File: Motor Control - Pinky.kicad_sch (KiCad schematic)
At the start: 9 parts, among them J4 BM09B-SRSS-TB, U12 TB9051FTG,EL

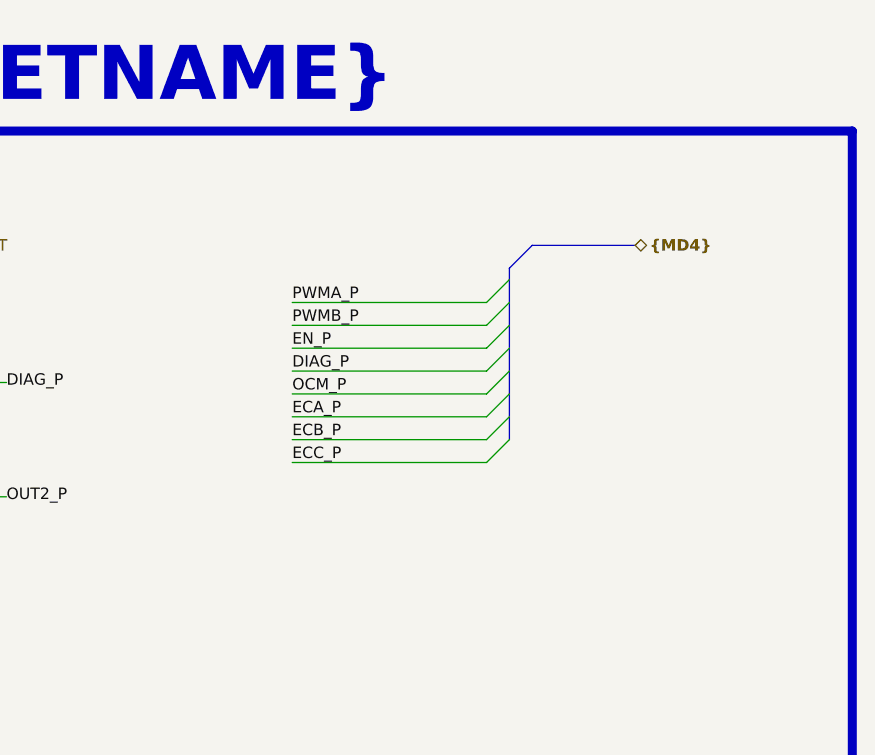
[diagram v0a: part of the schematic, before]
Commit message: Update Schematic
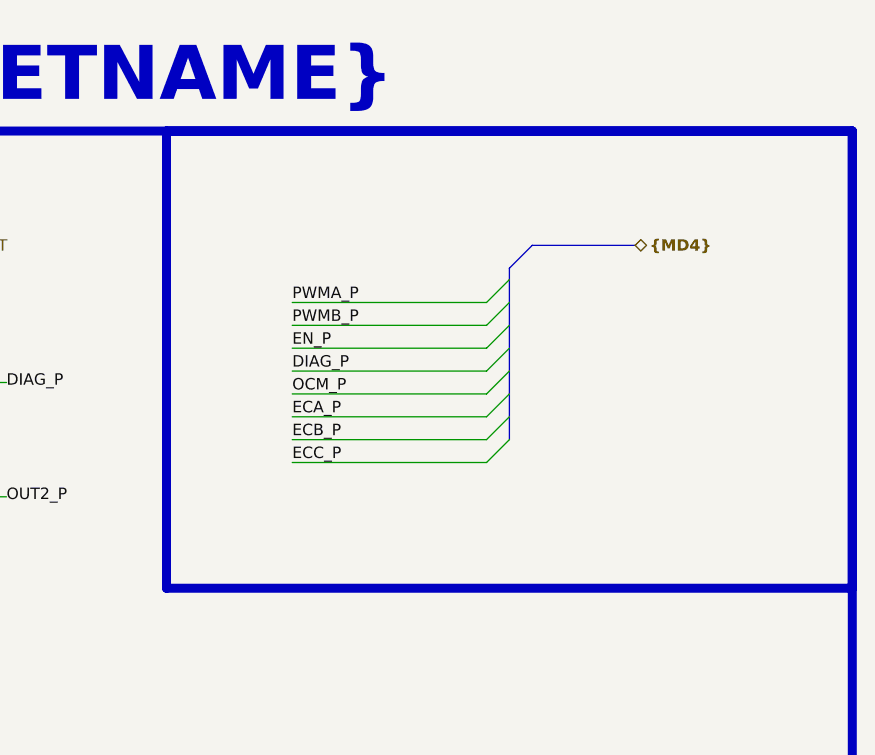
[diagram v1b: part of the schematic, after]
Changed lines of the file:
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@@
+		)
+	)
+	(rectangle
+		(start 177.8 25.4)
+		(end 254 76.2)
+		(stroke
+			(width 1)
+			(type default)
+			(color 200 0 0 1)
+		)
+		(fill
+			(type none)
 		)
 	)

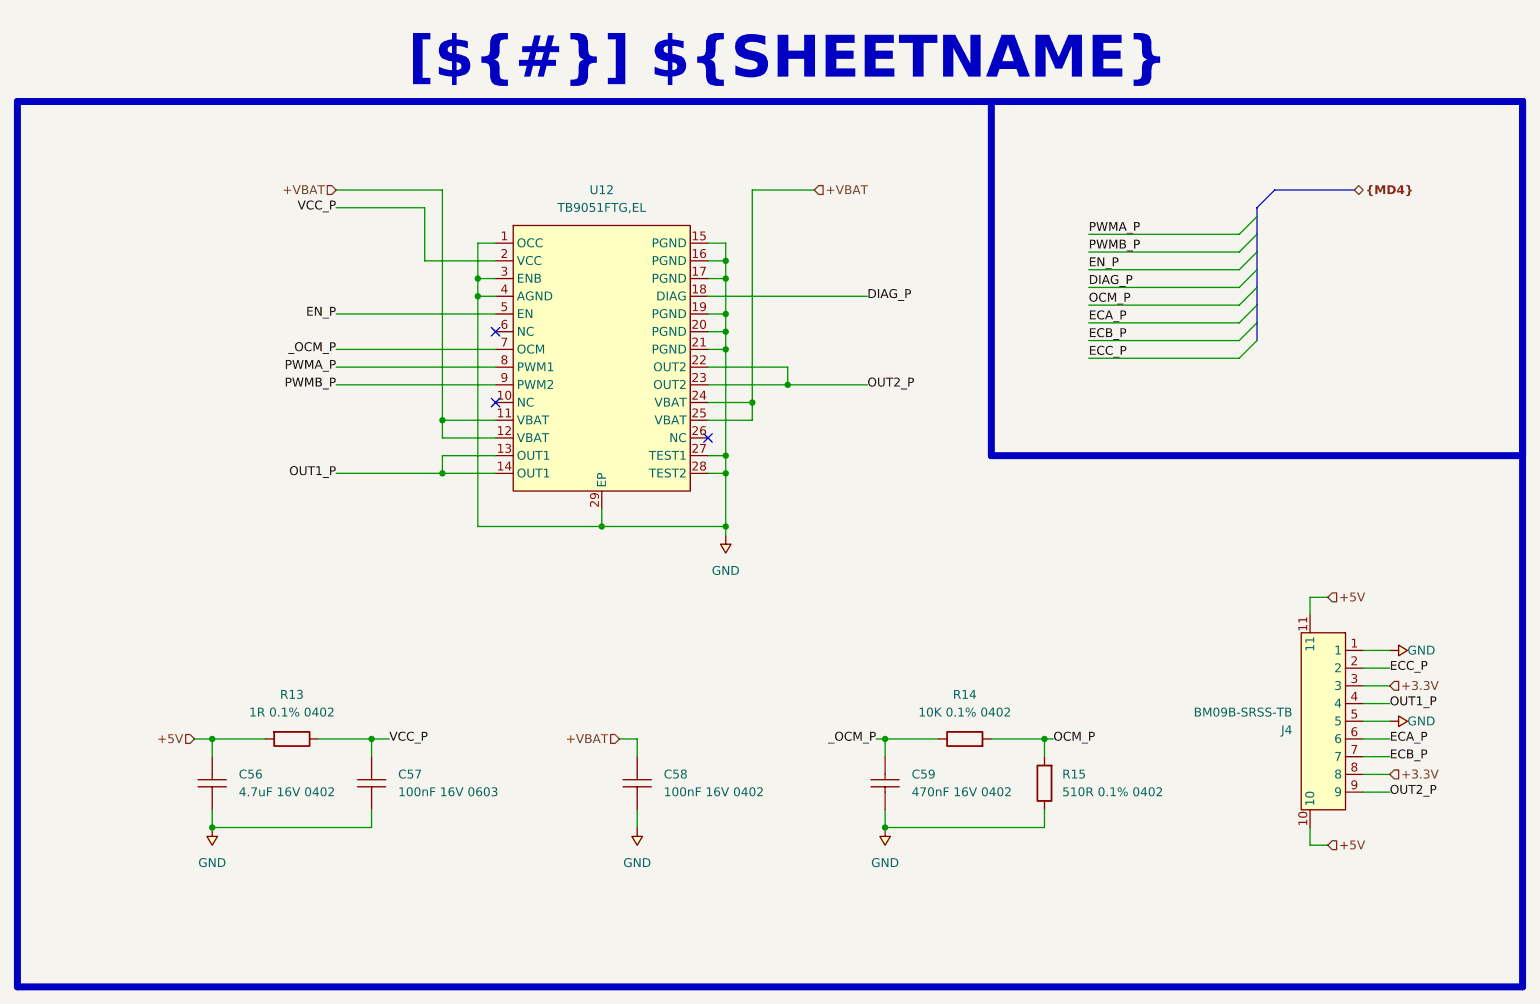
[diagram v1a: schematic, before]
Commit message: Update Schematic
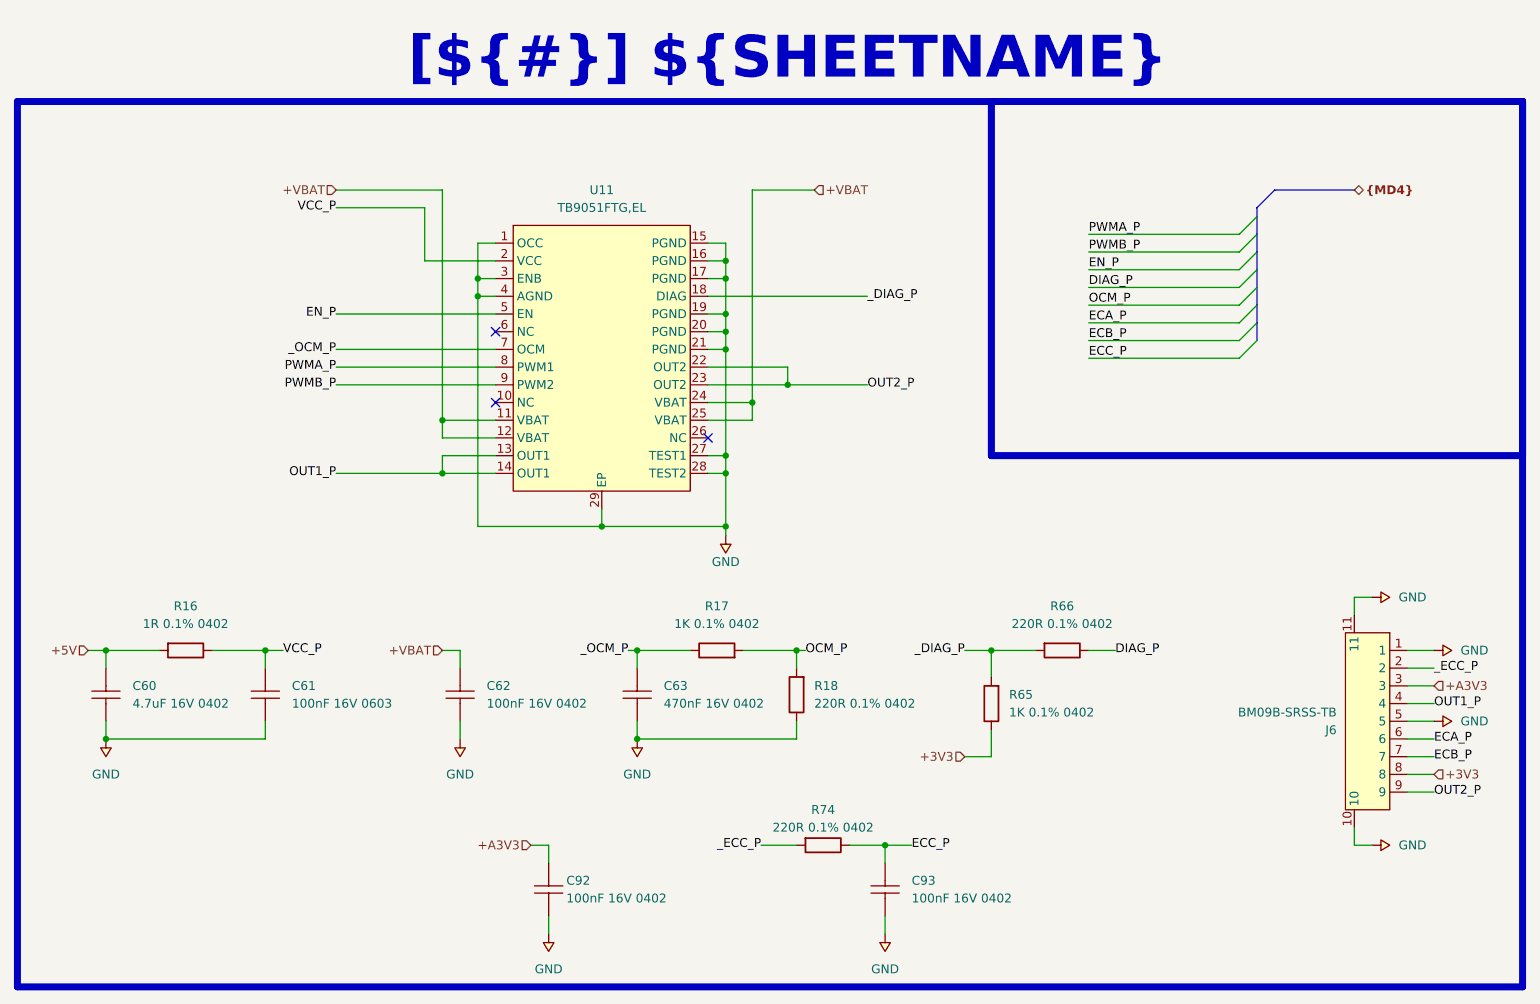
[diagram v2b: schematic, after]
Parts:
- removed J4: BM09B-SRSS-TB, Duc:CONN-SMD_9P-P1.00_BM09B-SRSS-TB, symbol Duc-Connectors:BM09B-SRSS-TB
- added C92, C93: 100nF 16V 0402, Duc_Library:C0402, symbol Duc-Capacitors:CAP CER 0402
- added J6: BM09B-SRSS-TB, Duc:CONN-SMD_9P-P1.00_BM09B-SRSS-TB, symbol Duc-Connectors:BM09B-SRSS-TB
- added R65: 1K 0.1% 0402, Duc_Library:R0402, symbol Duc-Resistors:RES SMD 0402
- added R66, R74: 220R 0.1% 0402, Duc_Library:R0402, symbol Duc-Resistors:RES SMD 0402
- R17: renamed from R14; value 10K 0.1% 0402 -> 1K 0.1% 0402
- R18: renamed from R15; value 510R 0.1% 0402 -> 220R 0.1% 0402
- renumbered C56 to C60, C57 to C61, C58 to C62, C59 to C63, R13 to R16, U12 to U11
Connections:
- net DIAG_P: now also R66.2; no longer U11.18 (DIAG)
- net ECA_P: now also J6.6
- net ECB_P: now also J6.7
- net ECC_P: now also C93.2, R74.2
- net GND: now also C92.1, C93.1, J6.1, J6.10, J6.11, J6.5
- net OUT1_P: now also J6.4
- net OUT2_P: now also J6.9
- new net +3V3: J6.8, R65.2
- new net +A3V3: C92.2, J6.3
- new net _DIAG_P: R65.1, R66.1, U11.18 (DIAG)
- new net _ECC_P: J6.2, R74.1
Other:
- moved on the sheet: C60, C61, C62, C63, R16, R17, R18
